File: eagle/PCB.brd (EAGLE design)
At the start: 100 x 80 mm, 24 parts, among them T1 2N2222, T2 2N2222

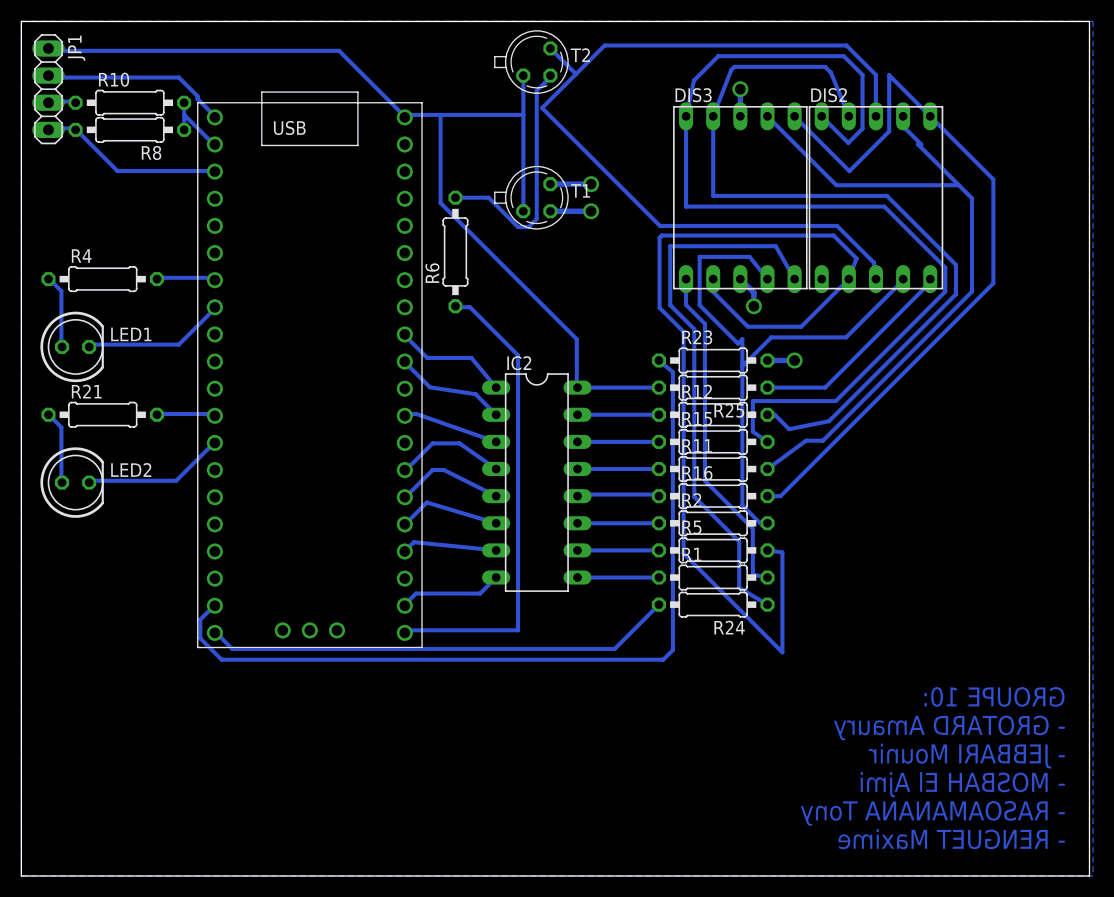
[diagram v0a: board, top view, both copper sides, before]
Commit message: Update PCB.brd
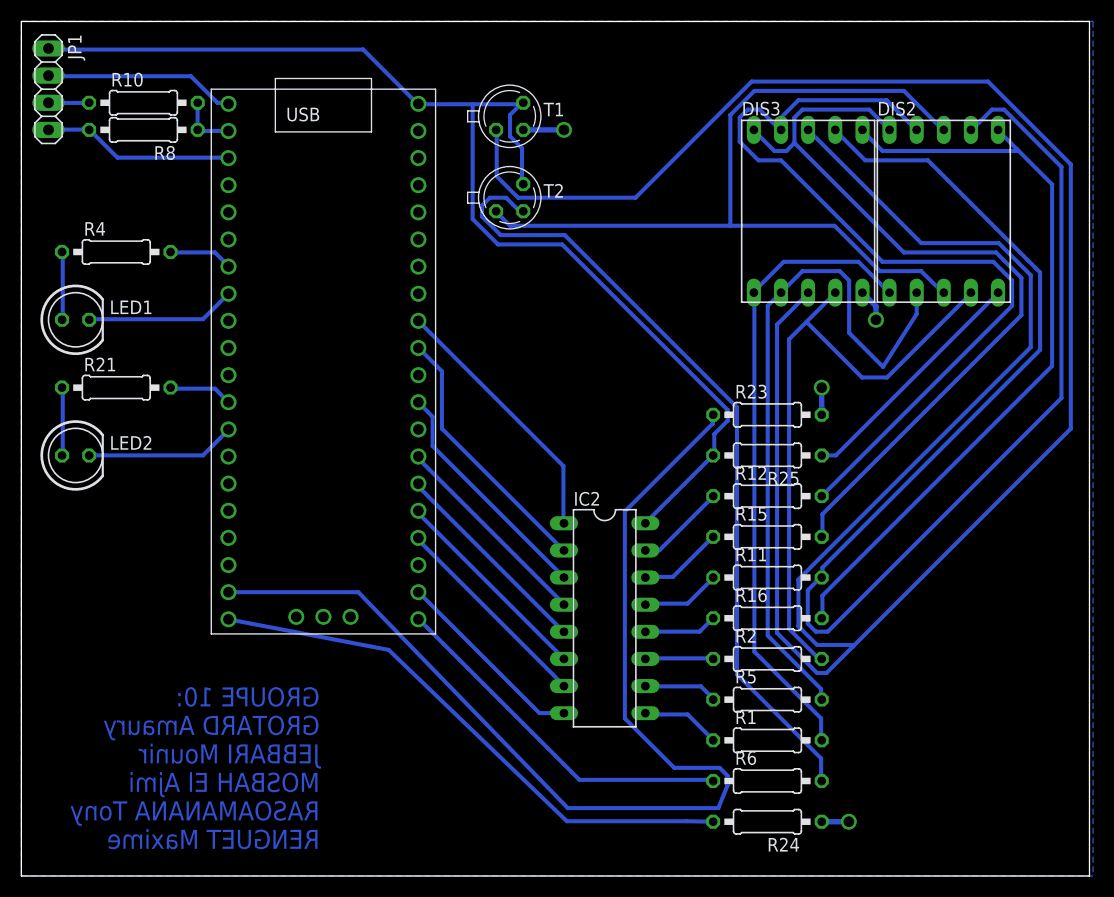
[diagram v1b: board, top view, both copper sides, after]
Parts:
- moved R6 57.5 mm to (69.8, 8.89), turned to 0 degrees
- moved R24 20.9 mm to (69.8, 5.08)
- moved R1 16.1 mm to (69.8, 12.7)
- moved R5 14.9 mm to (69.8, 16.5)
- moved IC2 14.2 mm to (54.6, 24.1)
- moved R2 13.7 mm to (69.8, 20.3)
- moved T2 13.0 mm to (45.7, 63.5)
- moved R16 12.5 mm to (69.8, 24.1)
- moved R11 11.4 mm to (69.8, 27.9)
- moved R15 10.2 mm to (69.8, 31.8)
- moved R12 9.16 mm to (69.8, 35.6)
- moved R25 8.13 mm to (69.8, 39.4)
- moved T1 8.03 mm to (45.7, 71.1)
- moved R23 7.18 mm to (69.8, 43.2)
- moved DIS2 6.48 mm to (86.4, 62.2)
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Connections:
- net N$25: now also T1.1; no longer T1.3
- net N$29: now also T2.1; no longer T2.3
- net VCC: now also T1.3, T2.3; no longer T1.1, T2.1
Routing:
- net N$25: track 9.42 -> 237.3 mm
- net 13A: track 65.9 -> 132.9 mm
- net N$30: track 23.0 -> 75.2 mm
- net N$33: track 51.2 -> 5.61 mm
- net 9E: track 31.7 -> 59.7 mm
- net 10D: track 92.9 -> 65.5 mm
- net 19TOTR: track 76.8 -> 101.3 mm
- net 14G: track 95.5 -> 75.8 mm
- net N$10: track 10.4 -> 24.6 mm
- net N$9: track 10.8 -> 24.6 mm
- net N$15: track 9.09 -> 22.0 mm
- net VCC: track 98.5 -> 111.1 mm
- net N$11: track 8.96 -> 19.5 mm
- net N$18: track 44.3 -> 33.9 mm
- net N$12: track 9.68 -> 19.5 mm
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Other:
- board text added: "GROUPE 10: GROTARD Amaury JEBBARI Mounir MOSBAH El Ajmi RASOAMANANA Tony RENGUET Maxime"
- board text removed: "GROUPE 10: - GROTARD Amaury - JEBBARI Mounir - MOSBAH El Ajmi - RASOAMANANA Tony - RENGUET Maxime"
